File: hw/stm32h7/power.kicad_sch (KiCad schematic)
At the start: 37 parts, among them J5 436500212, U5 LMR50410, U6 INA241A3xDDF, U7 TPS2116DRL, U8 TLV75733PDRV, U9 TLV75733PDRV

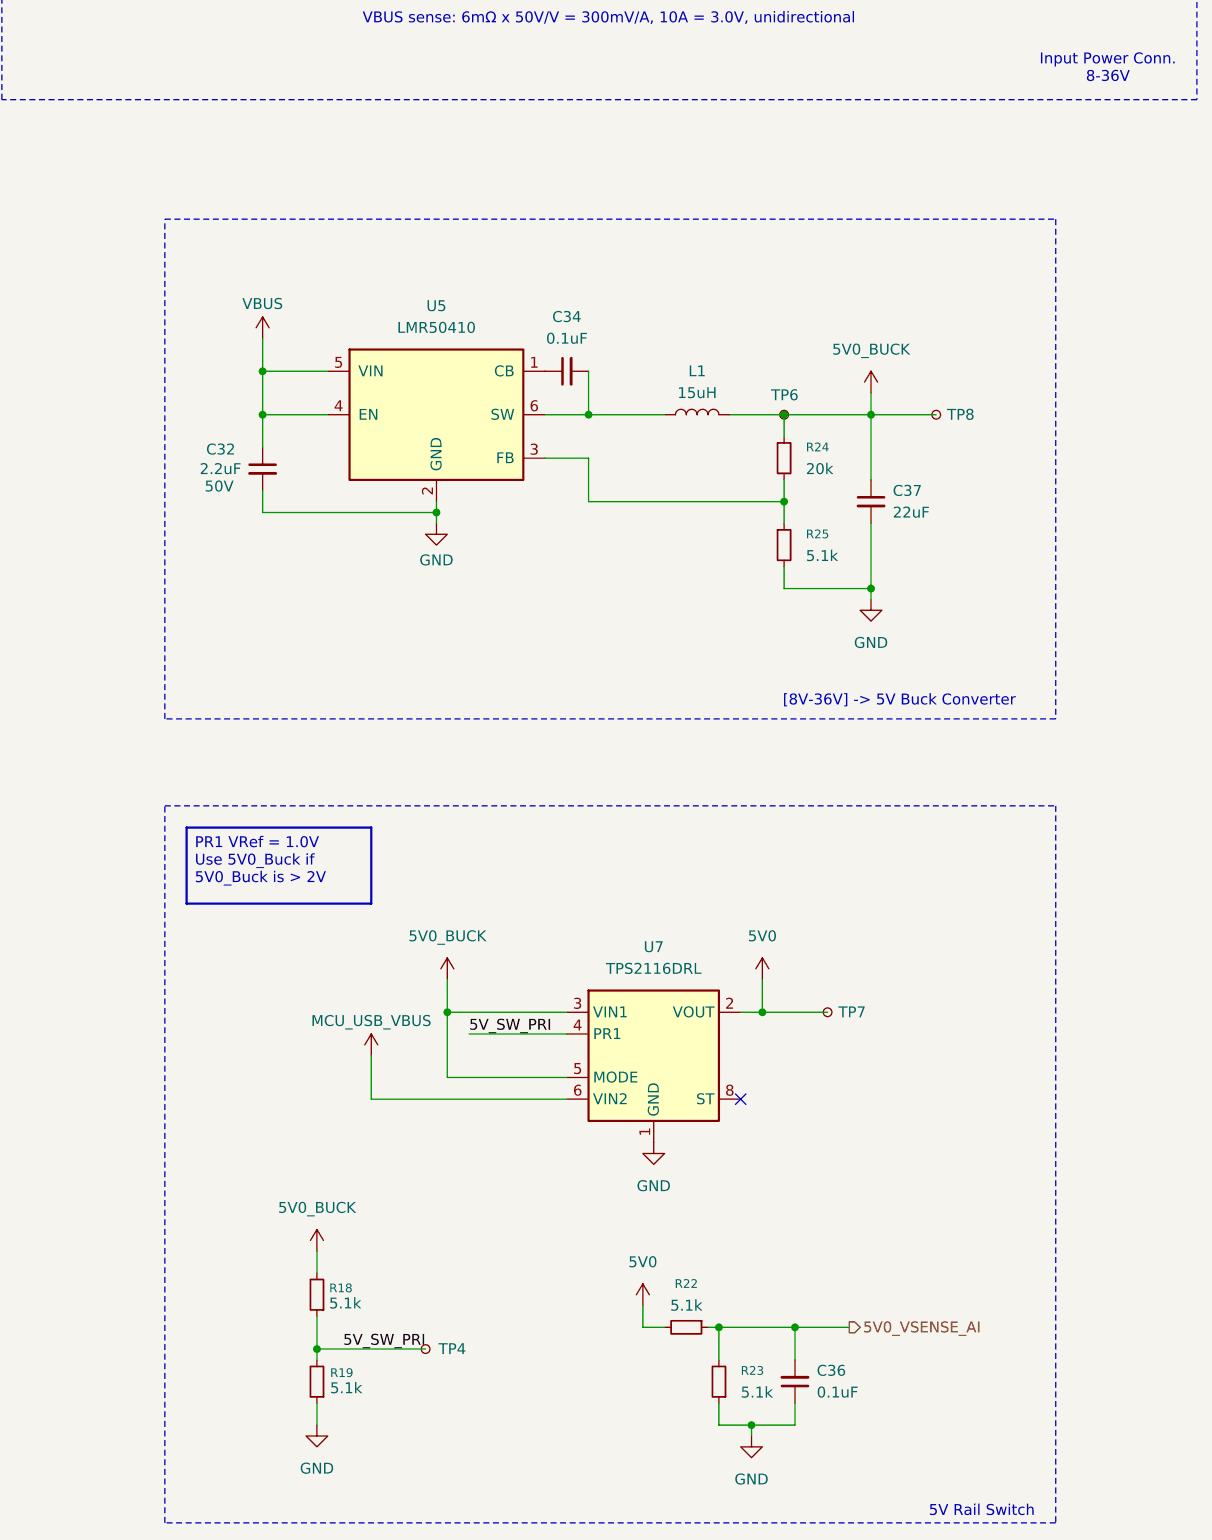
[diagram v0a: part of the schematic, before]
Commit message: WIP: schematic bringup
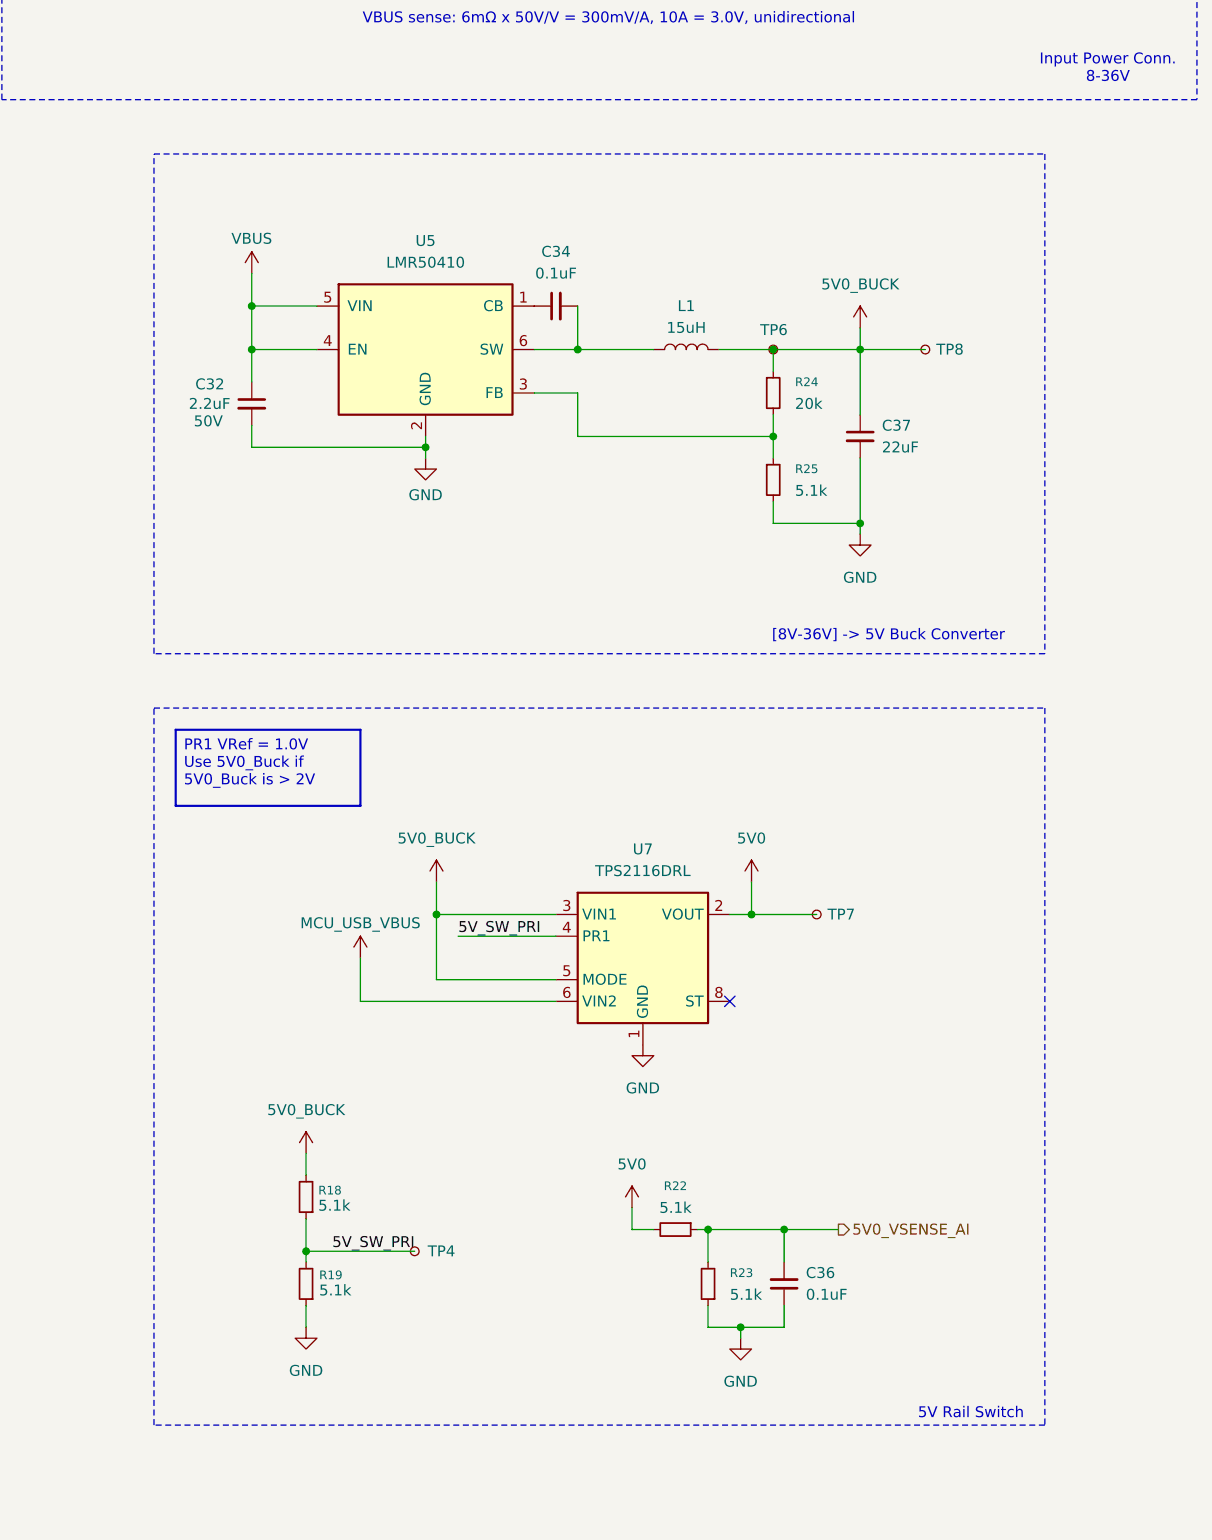
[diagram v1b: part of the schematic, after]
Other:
- moved on the sheet: C32, C34, C36, C37, L1, R18, R19, R22, R23, R24, R25, TP4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
